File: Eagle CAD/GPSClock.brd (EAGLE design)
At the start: 100 x 80 mm, 39 parts, among them IC3 LM1117, J1 AMP FCI 10103594-0001LF, J2 ISP, J3 POWER_JACKSUPER_BOMB_DIGITY, J4 BM06B-SRSS-TB, Q1 1A/60V/500mΩ, U1 CH340C, U3 AP2112-3.3V, U4 ATMEGA328P_TQFP, Y1 16MHz

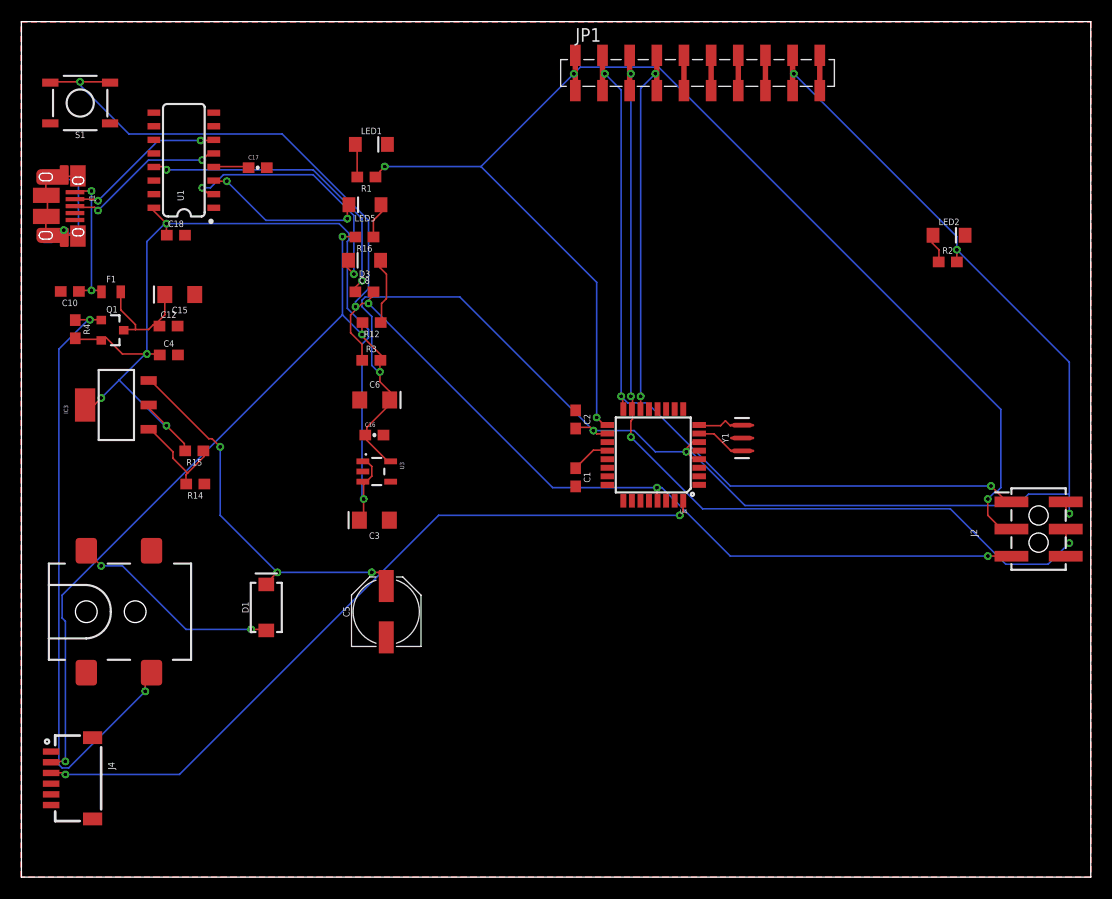
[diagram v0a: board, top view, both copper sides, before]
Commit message: Add files via upload
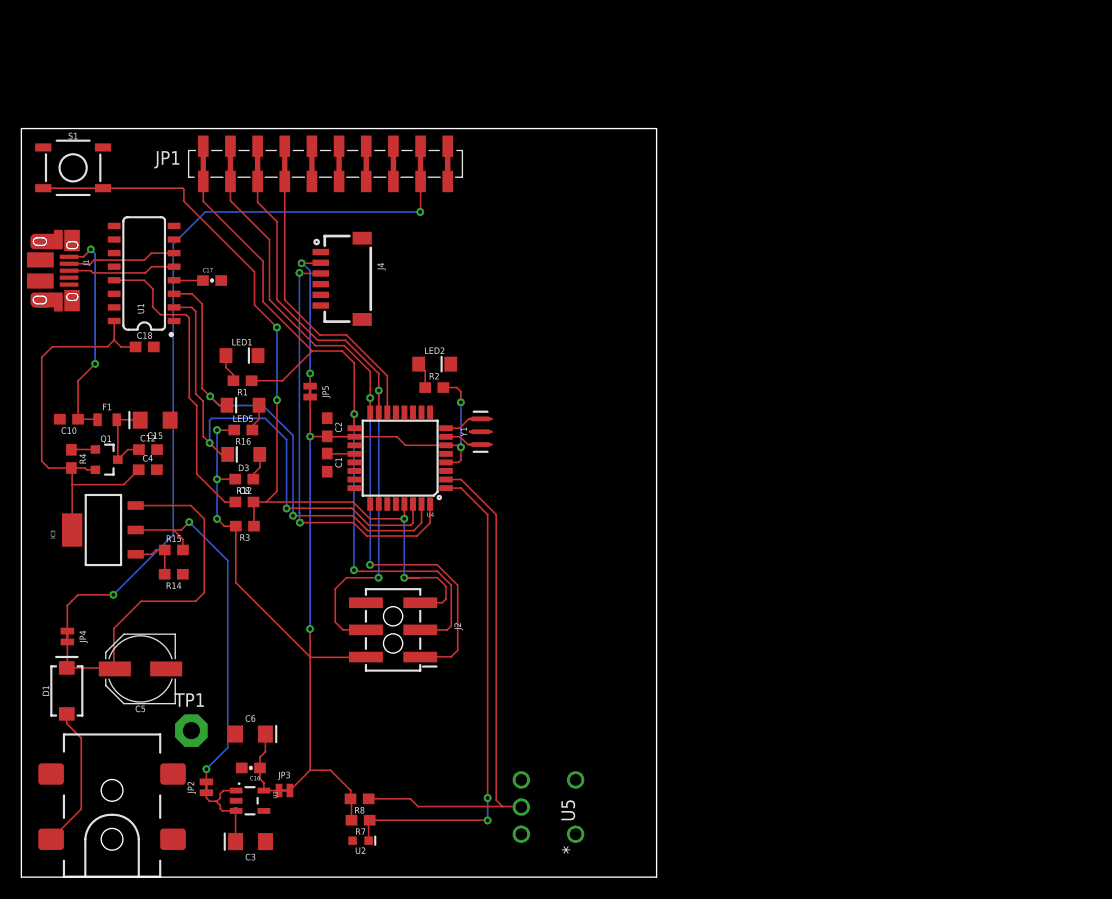
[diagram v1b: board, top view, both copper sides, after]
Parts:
- added JP2, JP3, JP4, JP5: JUMPER-SMT_2_NC_TRACE_NO-SILK, SparkFun-Jumpers:SMT-JUMPER_2_NC_TRACE_NO-SILK
- added R7: 1M, SparkFun-Resistors:0603
- added R8: 1k, SparkFun-Resistors:0603
- added TP1: TP-063, keystone:TP-063
- added U2: LIGHT_SENSORALS, SparkFun-Sensors:ALS-PT19
- added U5: 1571984-1, TE 1571984-1:SWITCH_1571984-1
- moved J2 61.1 mm to (34.8, 23.1), turned to 90 degrees
- moved J4 53.1 mm to (32.8, 56.0)
- moved LED2 49.6 mm to (38.6, 48.0)
- moved R2 49.4 mm to (38.6, 45.8)
- moved JP1 35.8 mm to (17.0, 66.7)
- moved C6 33.3 mm to (21.4, 13.4)
- moved C16 33.2 mm to (21.5, 10.2), turned to 180 degrees
- moved U3 33.0 mm to (21.4, 7.14)
- moved C3 32.2 mm to (21.4, 3.32)
- moved Y1 24.5 mm to (43.0, 41.6)
- moved U4 23.7 mm to (35.4, 39.2)
- moved C5 23.6 mm to (11.1, 19.5), turned to 180 degrees
- moved C1 23.3 mm to (28.6, 38.8)
- moved C2 23.2 mm to (28.6, 42.1)
- moved LED1 23.2 mm to (20.6, 48.8)
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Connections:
- net N$7 renamed GPS_RX
- new net AMBIENT: R7.1, U2.C, U4.1
- new net DTS: R8.1, U4.2, U5.5
- new net N$10: JP1.9A, JP1.9B, JP4.1
- new net N$11: J4.2, JP5.1
- new net N$7: C16.1, C6.+, JP3.1, U3.5
- new net N$8: JP2.1, U3.1, U3.3
- net 5V: now also JP2.2; no longer U3.1, U3.3
- net GND: now also TP1.1, U2.E, U5.1, U5.3, U5.6
- net RX-I: now also U4.30
- net TX-O: now also U4.31
- net VCC: now also JP3.2, JP5.2, R7.2, R8.2; no longer C16.1, C6.+, J4.2, JP1.9A, JP1.9B, U3.5
- net VIN: now also JP4.2
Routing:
- net VCC: track 229.8 -> 103.3 mm, vias 9 -> 7
- net N$10: track 0.00 -> 69.4 mm, vias 0 -> 2
- net INSERT: track 58.5 -> 2.25 mm, vias 2 -> 0
- net SCK: track 123.7 -> 68.6 mm, vias 4 -> 2
- net DTS: track 0.00 -> 48.2 mm
- net RESET: track 126.5 -> 79.7 mm, vias 5 -> 4
- net AMBIENT: track 0.00 -> 46.5 mm, vias 0 -> 2
- net MOSI: track 87.5 -> 56.1 mm, vias 4 -> 2
- net GPS_RX: track 70.4 -> 40.3 mm
- net TX-O: track 15.5 -> 45.3 mm
- net RX-I: track 24.7 -> 48.1 mm
- net SHLD: track 23.3 -> 0.00 mm, vias 1 -> 0
- net 5V: track 95.5 -> 76.2 mm, vias 5 -> 2
- net MISO: track 77.8 -> 63.0 mm, vias 3 -> 2
- net N$11: track 0.00 -> 13.7 mm, vias 0 -> 2
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- removed copper zone on layer 1, net GND
- removed copper zone on layer 16, net GND
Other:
- board size 100 x 80 mm -> 59.4 x 70 mm
- board text added: "Team 9: GPS Enabled Clock ECE 411 Fall 2019 Cheng, Jemmett, Jia & Liu"
